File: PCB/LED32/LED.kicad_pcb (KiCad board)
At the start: 2 copper layers, 32 x 32 mm, 179 parts, among them P1 Square, P2 Square, P3 Square

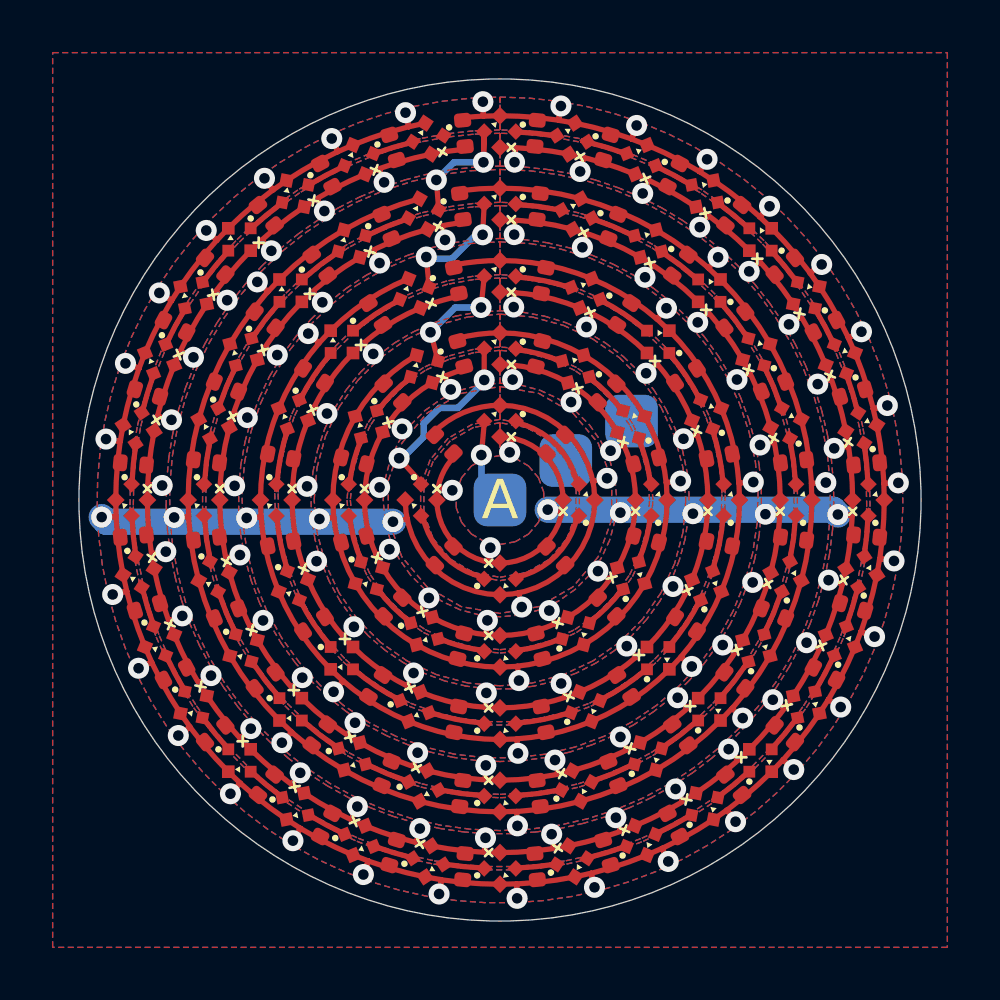
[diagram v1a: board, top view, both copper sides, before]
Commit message: Images
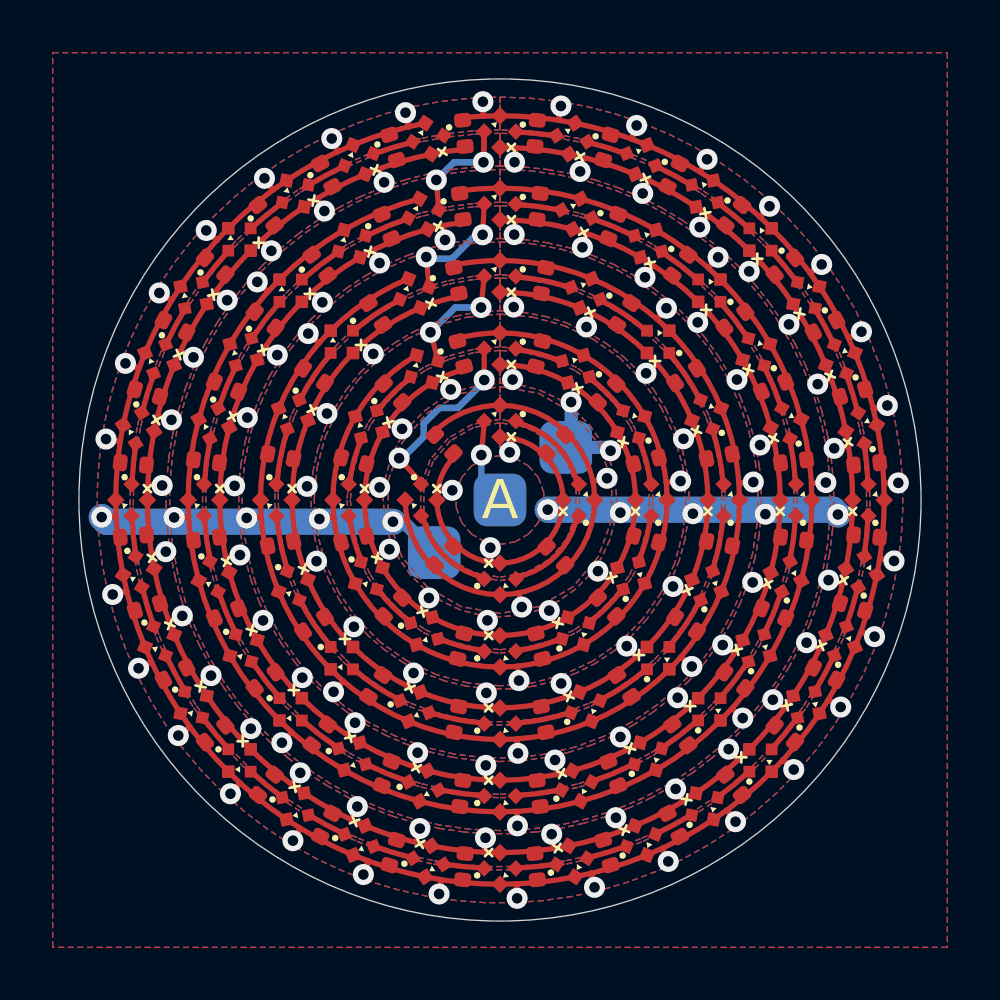
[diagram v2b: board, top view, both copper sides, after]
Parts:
- moved P3 6.10 mm to (97.5, 102.0)
- moved P1 2.69 mm to (102.5, 98.0)
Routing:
- net VCC: track 315.4 -> 318.7 mm
- net GND: track 333.2 -> 335.2 mm
